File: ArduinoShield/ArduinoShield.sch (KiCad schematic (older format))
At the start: 3 parts, among them J1 Conn_02x15_Odd_Even, J2 Conn_01x04

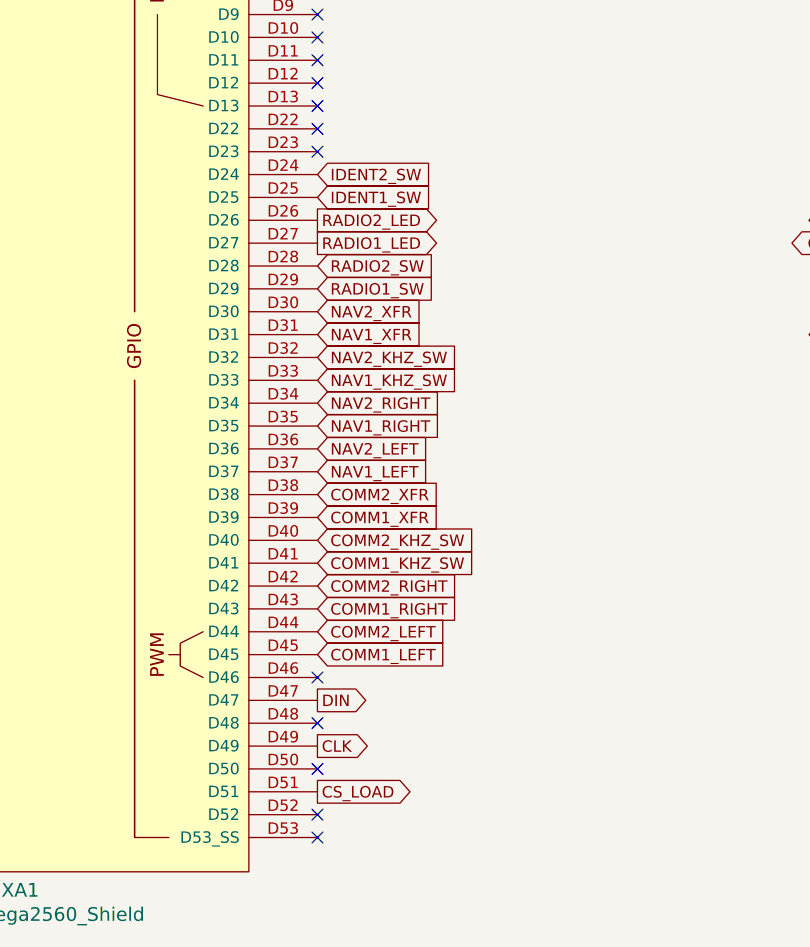
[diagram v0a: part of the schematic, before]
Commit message: Final version submitted for assembly
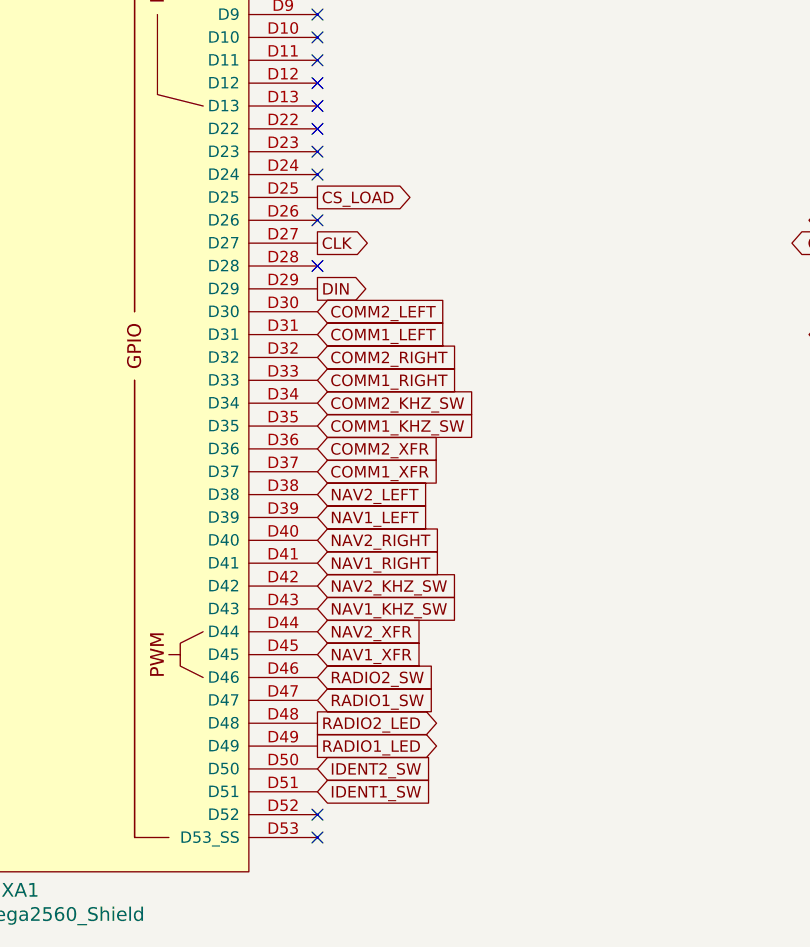
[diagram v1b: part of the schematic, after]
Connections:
- net CLK: now also XA1.D27; no longer XA1.D49
- net COMM1_KHZ_SW: now also XA1.D35; no longer XA1.D41
- net COMM1_LEFT: now also XA1.D31; no longer XA1.D45
- net COMM1_RIGHT: now also XA1.D33; no longer XA1.D43
- net COMM1_XFR: now also XA1.D37; no longer XA1.D39
- net COMM2_KHZ_SW: now also XA1.D34; no longer XA1.D40
- net COMM2_LEFT: now also XA1.D30; no longer XA1.D44
- net COMM2_RIGHT: now also XA1.D32; no longer XA1.D42
- net COMM2_XFR: now also XA1.D36; no longer XA1.D38
- net CS_LOAD: now also XA1.D25; no longer XA1.D51
- net DIN: now also XA1.D29; no longer XA1.D47
- net IDENT1_SW: now also XA1.D51; no longer XA1.D25
- net IDENT2_SW: now also XA1.D50; no longer XA1.D24
- net NAV1_KHZ_SW: now also XA1.D43; no longer XA1.D33
- net NAV1_LEFT: now also XA1.D39; no longer XA1.D37
- net NAV1_RIGHT: now also XA1.D41; no longer XA1.D35
- net NAV1_XFR: now also XA1.D45; no longer XA1.D31
- net NAV2_KHZ_SW: now also XA1.D42; no longer XA1.D32
- net NAV2_LEFT: now also XA1.D38; no longer XA1.D36
- net NAV2_RIGHT: now also XA1.D40; no longer XA1.D34
- net NAV2_XFR: now also XA1.D44; no longer XA1.D30
- net RADIO1_LED: now also XA1.D49; no longer XA1.D27
- net RADIO1_SW: now also XA1.D47; no longer XA1.D29
- net RADIO2_LED: now also XA1.D48; no longer XA1.D26
- net RADIO2_SW: now also XA1.D46; no longer XA1.D28
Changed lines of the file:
@@
 NoConn ~ 2100 4650
 NoConn ~ 2100 4750
-Text GLabel 4700 5250 2    50   Output ~ 0
+Text GLabel 4700 3450 2    50   Output ~ 0
 DIN
-Text GLabel 4700 5650 2    50   Output ~ 0
+Text GLabel 4700 3050 2    50   Output ~ 0
 CS_LOAD
-Text GLabel 4700 5450 2    50   Output ~ 0
+Text GLabel 4700 3250 2    50   Output ~ 0
 CLK
 Text GLabel 7450 2950 0    50   Input ~ 0
@@
 Text GLabel 7450 3250 0    50   Output ~ 0
 COMM1_KHZ_SW
-Text GLabel 4700 4650 2    50   Input ~ 0
+Text GLabel 4700 4050 2    50   Input ~ 0
 COMM1_KHZ_SW
 Text GLabel 7450 3050 0    50   Output ~ 0
@@
 Text GLabel 7450 3150 0    50   Output ~ 0
 COMM1_RIGHT
-Text GLabel 4700 5050 2    50   Input ~ 0
+Text GLabel 4700 3650 2    50   Input ~ 0
 COMM1_LEFT
-Text GLabel 4700 4850 2    50   Input ~ 0
+Text GLabel 4700 3850 2    50   Input ~ 0
 COMM1_RIGHT
 Text GLabel 7450 3450 0    50   Output ~ 0
@@
 Text GLabel 7450 3650 0    50   Output ~ 0
 NAV1_KHZ_SW
-Text GLabel 4700 4250 2    50   Input ~ 0
+Text GLabel 4700 4450 2    50   Input ~ 0
 NAV1_LEFT
-Text GLabel 4700 4050 2    50   Input ~ 0
+Text GLabel 4700 4650 2    50   Input ~ 0
 NAV1_RIGHT
-Text GLabel 4700 3850 2    50   Input ~ 0
+Text GLabel 4700 4850 2    50   Input ~ 0
 NAV1_KHZ_SW
 Text GLabel 7450 3850 0    50   Output ~ 0
 RADIO1_SW
-Text GLabel 4700 3450 2    50   Input ~ 0
+Text GLabel 4700 5250 2    50   Input ~ 0
 RADIO1_SW
 Text GLabel 7950 3050 2    50   Output ~ 0
@@
 Text GLabel 7950 3250 2    50   Output ~ 0
 COMM2_KHZ_SW
-Text GLabel 4700 4950 2    50   Input ~ 0
+Text GLabel 4700 3550 2    50   Input ~ 0
 COMM2_LEFT
-Text GLabel 4700 4750 2    50   Input ~ 0
+Text GLabel 4700 3750 2    50   Input ~ 0
 COMM2_RIGHT
-Text GLabel 4700 4550 2    50   Input ~ 0
+Text GLabel 4700 3950 2    50   Input ~ 0
 COMM2_KHZ_SW
 $Comp
@@
 Text GLabel 7450 3750 0    50   Output ~ 0
 NAV1_XFR
+Text GLabel 4700 4350 2    50   Input ~ 0
+NAV2_LEFT
+Text GLabel 4700 4550 2    50   Input ~ 0
+NAV2_RIGHT
+Text GLabel 4700 4750 2    50   Input ~ 0
+NAV2_KHZ_SW
 Text GLabel 4700 4150 2    50   Input ~ 0
-NAV2_LEFT
-Text GLabel 4700 3950 2    50   Input ~ 0
-NAV2_RIGHT
-Text GLabel 4700 3750 2    50   Input ~ 0
-NAV2_KHZ_SW
-Text GLabel 4700 4350 2    50   Input ~ 0
 COMM2_XFR
-Text GLabel 4700 4450 2    50   Input ~ 0
+Text GLabel 4700 4250 2    50   Input ~ 0
 COMM1_XFR
 Text GLabel 7950 3450 2    50   Output ~ 0
@@
 Text GLabel 7950 3750 2    50   Output ~ 0
 NAV2_XFR
-Text GLabel 4700 3550 2    50   Input ~ 0
+Text GLabel 4700 4950 2    50   Input ~ 0
 NAV2_XFR
-Text GLabel 4700 3650 2    50   Input ~ 0
+Text GLabel 4700 5050 2    50   Input ~ 0
 NAV1_XFR
-Text GLabel 4700 3350 2    50   Input ~ 0
+Text GLabel 4700 5150 2    50   Input ~ 0
 RADIO2_SW
 Text GLabel 7950 3850 2    50   Output ~ 0
@@
 Text GLabel 7950 4050 2    50   Output ~ 0
 IDENT2_SW
-Text GLabel 4700 3050 2    50   Input ~ 0
+Text GLabel 4700 5650 2    50   Input ~ 0
 IDENT1_SW
-Text GLabel 4700 2950 2    50   Input ~ 0
+Text GLabel 4700 5550 2    50   Input ~ 0
 IDENT2_SW
 Text GLabel 7450 4050 0    50   Output ~ 0
@@
 Text GLabel 7950 3950 2    50   Input ~ 0
 RADIO2_LED
-Text GLabel 4700 3150 2    50   Output ~ 0
+Text GLabel 4700 5350 2    50   Output ~ 0
 RADIO2_LED
-Text GLabel 4700 3250 2    50   Output ~ 0
+Text GLabel 4700 5450 2    50   Output ~ 0
 RADIO1_LED
 $Comp
@@
 	1    0    0    -1
 $EndComp
-NoConn ~ 4700 5750
-NoConn ~ 4700 5850
 $Comp
 L power:PWR_FLAG #FLG0101
@@
 	1    0    0    -1
 $EndComp
-NoConn ~ 4700 5150
-NoConn ~ 4700 5350
 NoConn ~ 4700 2850
-NoConn ~ 4700 5550
+NoConn ~ 4700 3150
+NoConn ~ 4700 2950
+NoConn ~ 4700 3350
+NoConn ~ 4700 5750
+NoConn ~ 4700 5850
 $EndSCHEMATC
